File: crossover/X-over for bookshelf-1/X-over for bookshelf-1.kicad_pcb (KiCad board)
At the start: 2 copper layers, 10 parts, among them J1 Screw_Terminal_01x02, J2 Screw_Terminal_01x04

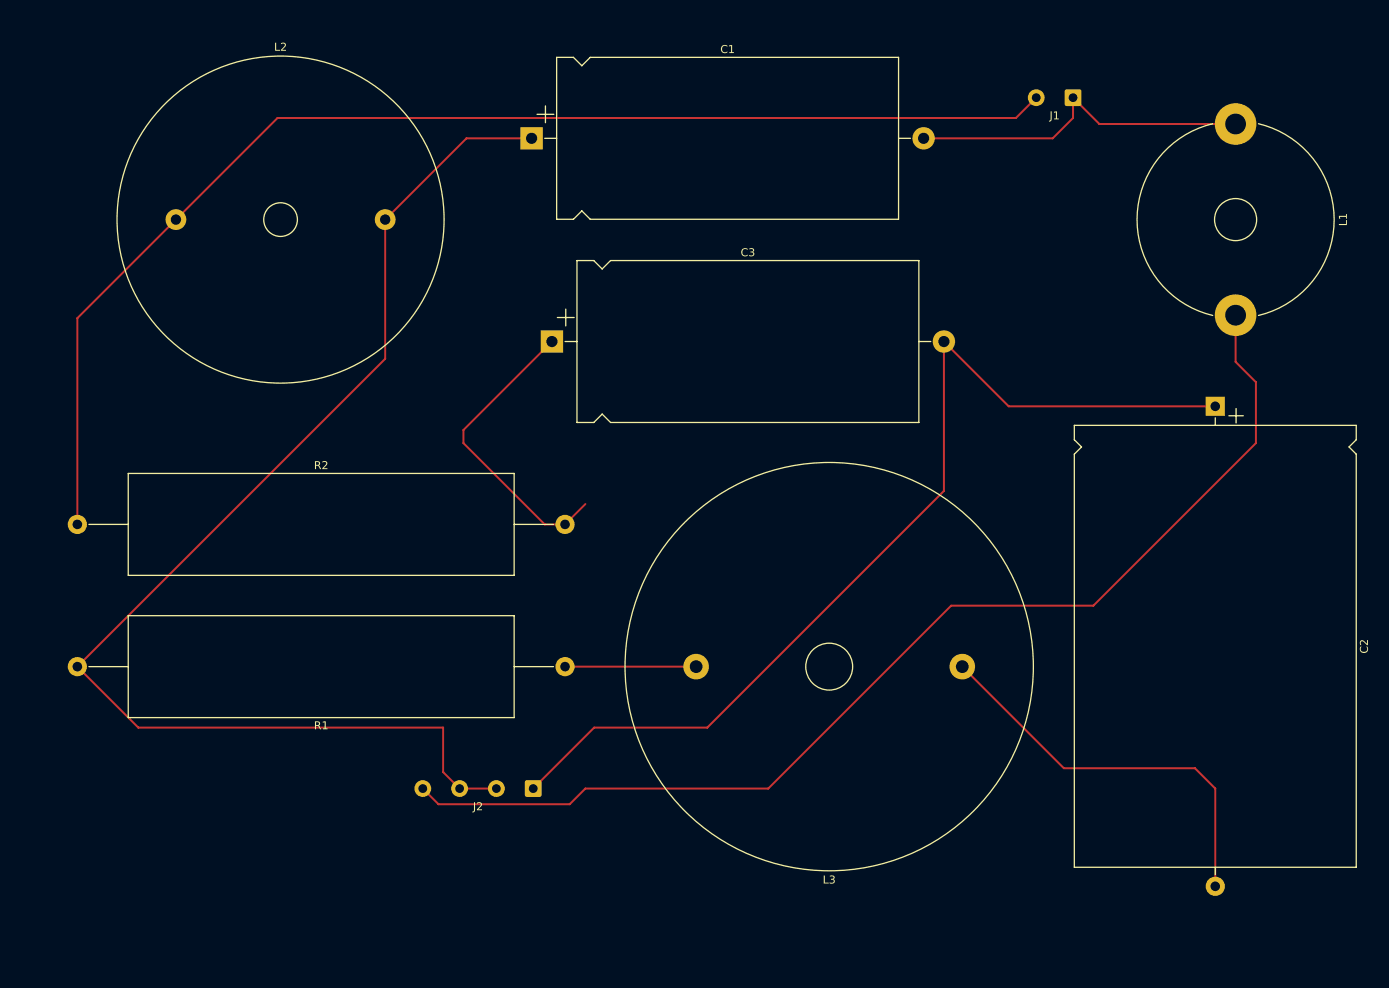
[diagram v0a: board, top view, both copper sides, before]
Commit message: adding KiCAD documents for the XO design
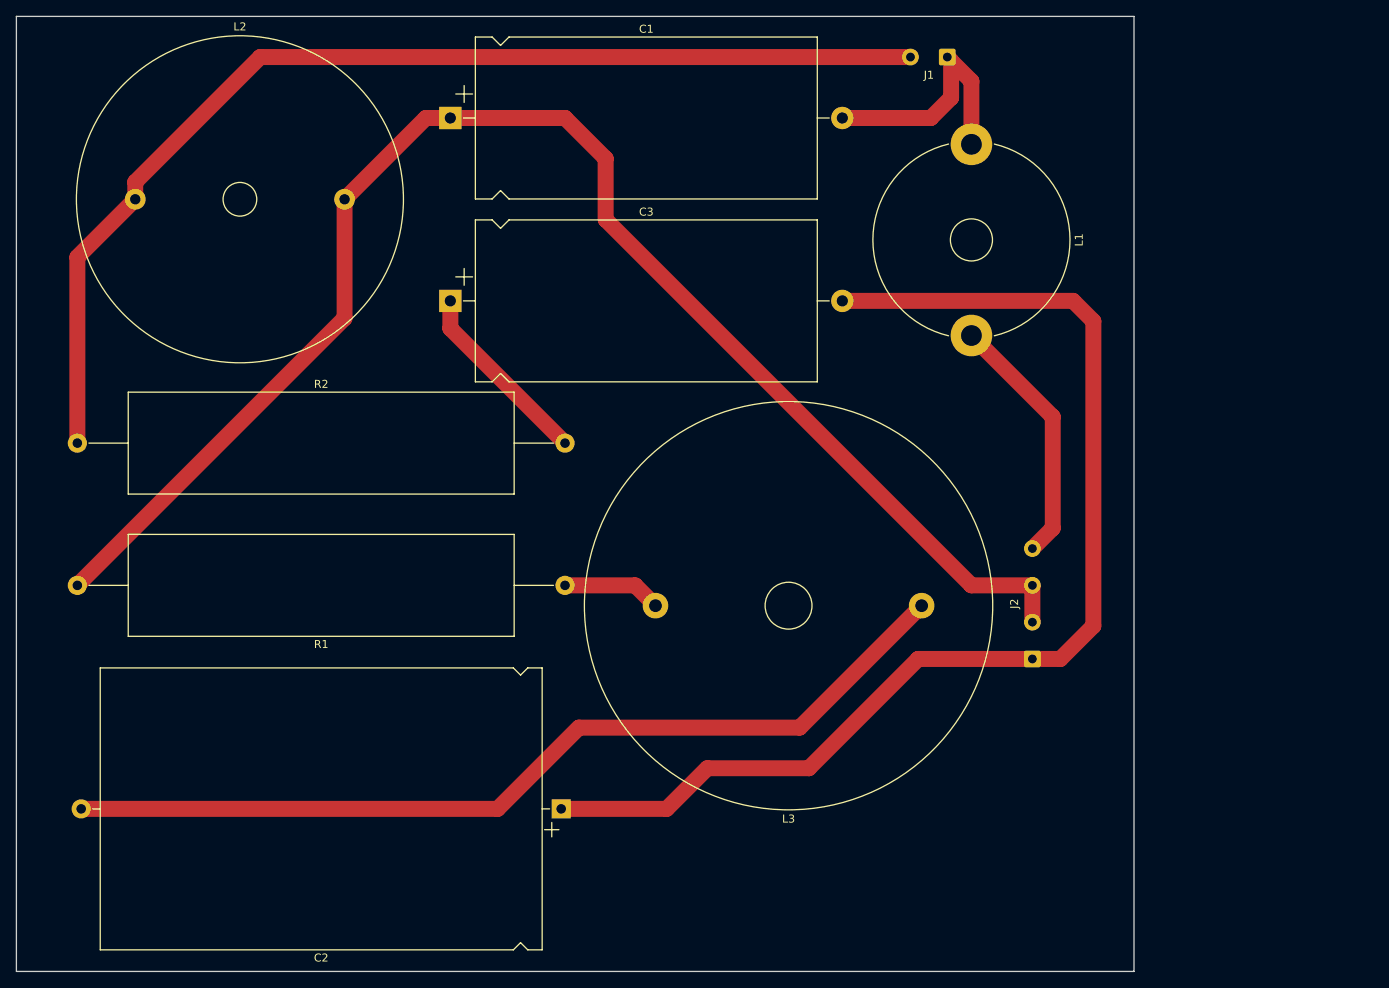
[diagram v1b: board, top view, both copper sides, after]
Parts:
- moved C2 96.0 mm to (134.1, 132.1), turned to 180 degrees
- moved J2 64.5 mm to (193.0, 113.3), turned to 90 degrees
- moved L1 33.1 mm to (185.4, 49.0)
- moved J1 16.5 mm to (182.4, 38.1)
- moved C3 13.7 mm to (120.3, 68.6)
- moved C1 10.5 mm to (120.3, 45.7)
- moved R1 10.2 mm to (134.6, 104.1)
- moved R2 10.2 mm to (73.7, 86.4)
- moved L3 9.16 mm to (179.2, 106.7)
- moved L2 5.68 mm to (80.9, 55.9)
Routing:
- net Net-(J2-Pin_4): track 140.7 -> 31.9 mm
- net Net-(C2-Pad2): track 50.2 -> 115.6 mm
- net Net-(J2-Pin_2): track 156.3 -> 185.5 mm
- net Net-(J2-Pin_1): track 122.7 -> 146.5 mm
- net Net-(J1-Pin_2): track 157.1 -> 139.0 mm
- net Net-(J1-Pin_1): track 46.5 -> 32.1 mm
- net Net-(C3-Pad1): track 37.8 -> 23.7 mm
- net Net-(L3-Pad2): track 16.4 -> 12.4 mm
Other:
- board outline added: 139.7 x 119.4 mm
